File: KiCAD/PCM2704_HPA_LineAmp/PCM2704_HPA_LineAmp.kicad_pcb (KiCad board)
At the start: 2 copper layers, 33 parts, among them J1 HPA_L, J10 PCM2704Board, J11 USB_LED, J2 LINE_L, J3 HPA_R, J4 LINE_R, J5 PWR_IN, J6 PWR_OUT, J7 PWR_OUT, J8 TP_GND, J9 PWR_LED, U1 NJM4580

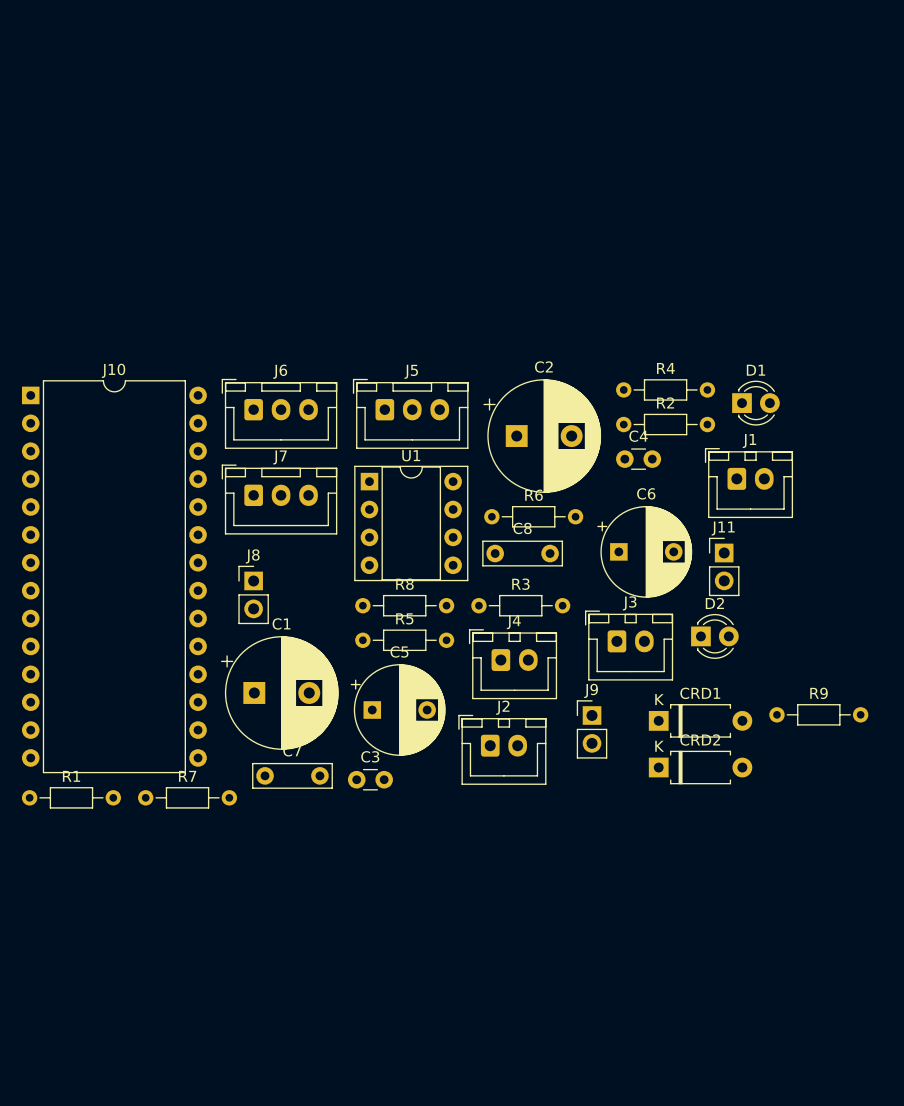
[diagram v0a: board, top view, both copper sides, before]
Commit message: Update: PCM2704_HPA_LineAmp board design
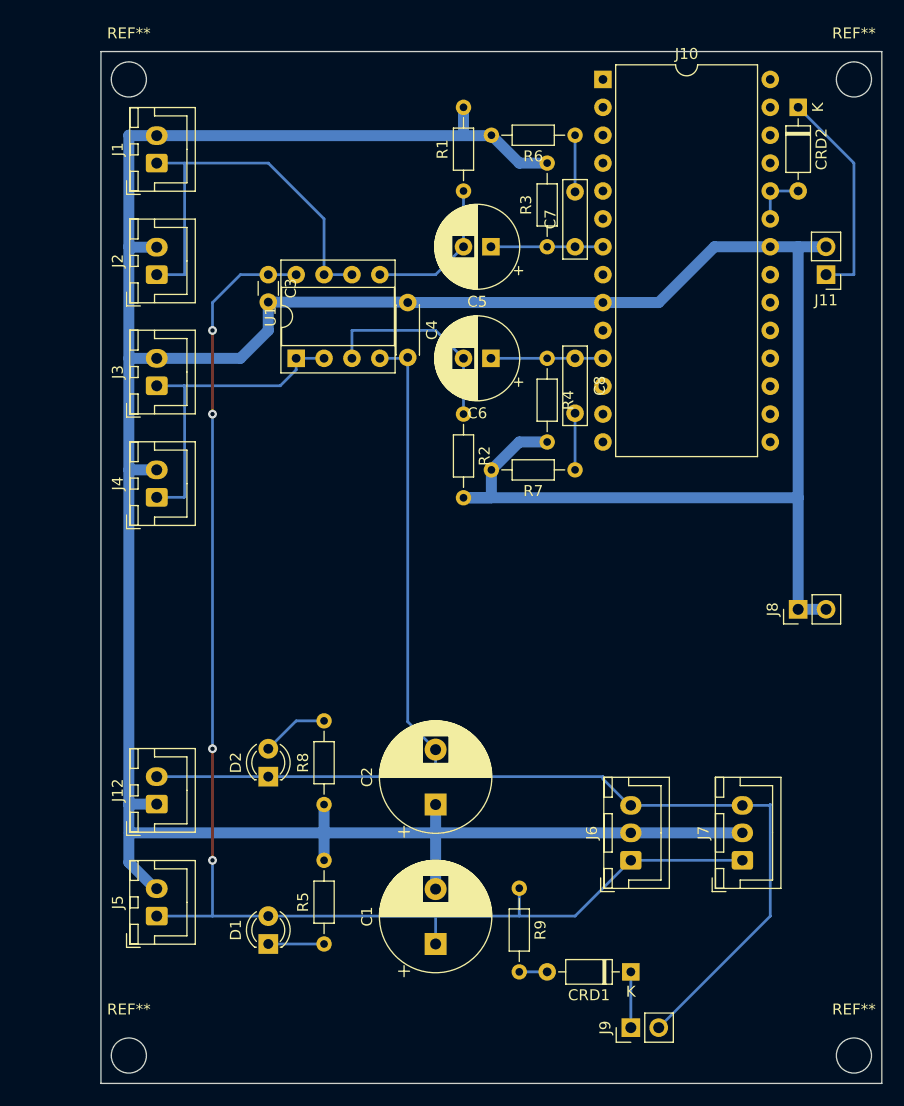
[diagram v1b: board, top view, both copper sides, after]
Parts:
- added J12: PWR-, Connector_JST:JST_XH_B2B-XH-A_1x02_P2.50mm_Vertical, F.Cu at (119.4, 114.3)
- added REF**: MountingHole_3.2mm_M3, MountingHole:MountingHole_3.2mm_M3, F.Cu at (116.8, 48.3)
- added REF**: MountingHole_3.2mm_M3, MountingHole:MountingHole_3.2mm_M3, F.Cu at (182.9, 48.3)
- added REF**: MountingHole_3.2mm_M3, MountingHole:MountingHole_3.2mm_M3, F.Cu at (182.9, 137.2)
- added REF**: MountingHole_3.2mm_M3, MountingHole:MountingHole_3.2mm_M3, F.Cu at (116.8, 137.2)
- C4: footprint Capacitor_THT:C_Disc_D3.0mm_W1.6mm_P2.50mm -> Capacitor_THT:C_Disc_D4.3mm_W1.9mm_P5.00mm
- C5, C6: footprint Capacitor_THT:CP_Radial_D8.0mm_P5.00mm -> Capacitor_THT:CP_Radial_D7.5mm_P2.50mm
- CRD1, CRD2: footprint Diode_THT:D_A-405_P7.62mm_Horizontal -> Diode_THT:D_DO-35_SOD27_P7.62mm_Horizontal
- J5: value PWR_IN -> PWR+; footprint Connector_JST:JST_XH_B3B-XH-A_1x03_P2.50mm_Vertical -> Connector_JST:JST_XH_B2B-XH-A_1x02_P2.50mm_Vertical
- moved R1 67.9 mm to (147.3, 58.4), turned to 90 degrees
- moved D1 65.5 mm to (129.5, 127.0), turned to 90 degrees
- moved CRD2 61.5 mm to (177.8, 50.8), turned to 270 degrees
- moved J1 60.2 mm to (119.4, 55.9), turned to 90 degrees
- moved J10 59.5 mm to (160.0, 48.3)
- moved C7 55.9 mm to (157.5, 63.5), turned to 90 degrees
- moved J7 55.6 mm to (172.7, 119.4), turned to 90 degrees
- moved J6 53.5 mm to (162.6, 119.4), turned to 90 degrees
- moved J2 52.6 mm to (119.4, 66.0), turned to 90 degrees
- moved J5 50.6 mm to (119.4, 124.5), turned to 90 degrees
- moved J8 49.7 mm to (177.8, 96.5), turned to 90 degrees
- moved R7 49.2 mm to (157.5, 83.8), turned to 180 degrees
- moved J3 47.9 mm to (119.4, 76.2), turned to 90 degrees
- moved C3 46.7 mm to (129.5, 66.0), turned to 270 degrees
- moved C5 43.6 mm to (149.8, 63.5), turned to 180 degrees
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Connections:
- D1 pad 1: GND -> Net-(D1-Pad1)
- D1 pad 2: Net-(D1-Pad2) -> +9V
- R5 pad 1: +9V -> Net-(D1-Pad1)
- R5 pad 2: Net-(D1-Pad2) -> GND
- U1 pad 1: Net-(J1-Pad1) -> Net-(J3-Pad1)
- U1 pad 2: Net-(J1-Pad1) -> Net-(J3-Pad1)
- U1 pad 3: Net-(C5-Pad2) -> Net-(C6-Pad2)
- U1 pad 5: Net-(C6-Pad2) -> Net-(C5-Pad2)
- U1 pad 6: Net-(J3-Pad1) -> Net-(J1-Pad1)
- U1 pad 7: Net-(J3-Pad1) -> Net-(J1-Pad1)
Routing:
- net GND: track 0.00 -> 334.4 mm
- net +9V: track 0.00 -> 125.1 mm, vias 0 -> 4
- net -9V: track 0.00 -> 123.5 mm
- net Net-(J1-Pad1): track 0.00 -> 37.7 mm
- net Net-(J3-Pad1): track 0.00 -> 29.6 mm
- net Net-(CRD2-Pad1): track 0.00 -> 19.9 mm
- net Net-(C6-Pad2): track 0.00 -> 18.8 mm
- net Net-(C5-Pad2): track 0.00 -> 13.8 mm
- net Net-(C6-Pad1): track 0.00 -> 10.2 mm
- net Net-(C5-Pad1): track 0.00 -> 10.2 mm
- net Net-(D2-Pad2): track 0.00 -> 6.13 mm
- net Net-(C8-Pad2): track 0.00 -> 5.16 mm
- net Net-(C7-Pad2): track 0.00 -> 5.16 mm
- net +5V: track 0.00 -> 5.08 mm
- net Net-(D1-Pad1): track 0.00 -> 5.08 mm
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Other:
- board outline added: 71.1 x 94 mm
